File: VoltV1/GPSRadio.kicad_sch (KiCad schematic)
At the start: 13 parts, among them J3 Conn_Coaxial, J4 Conn_Coaxial, U3 MAX-M10S-00B, U9 E22-900M30S

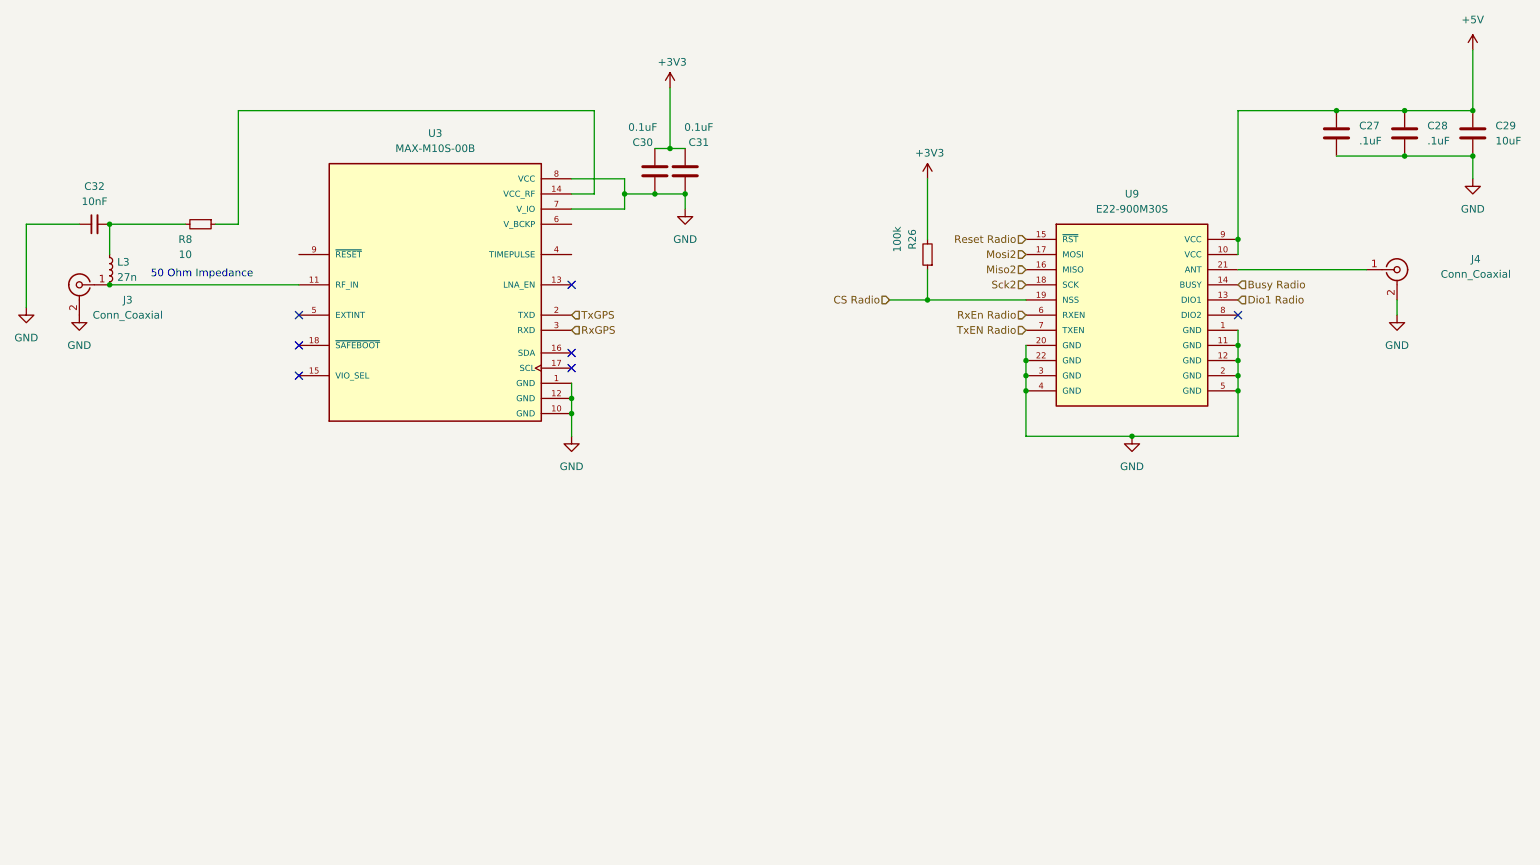
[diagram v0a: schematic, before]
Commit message: updates to schematic
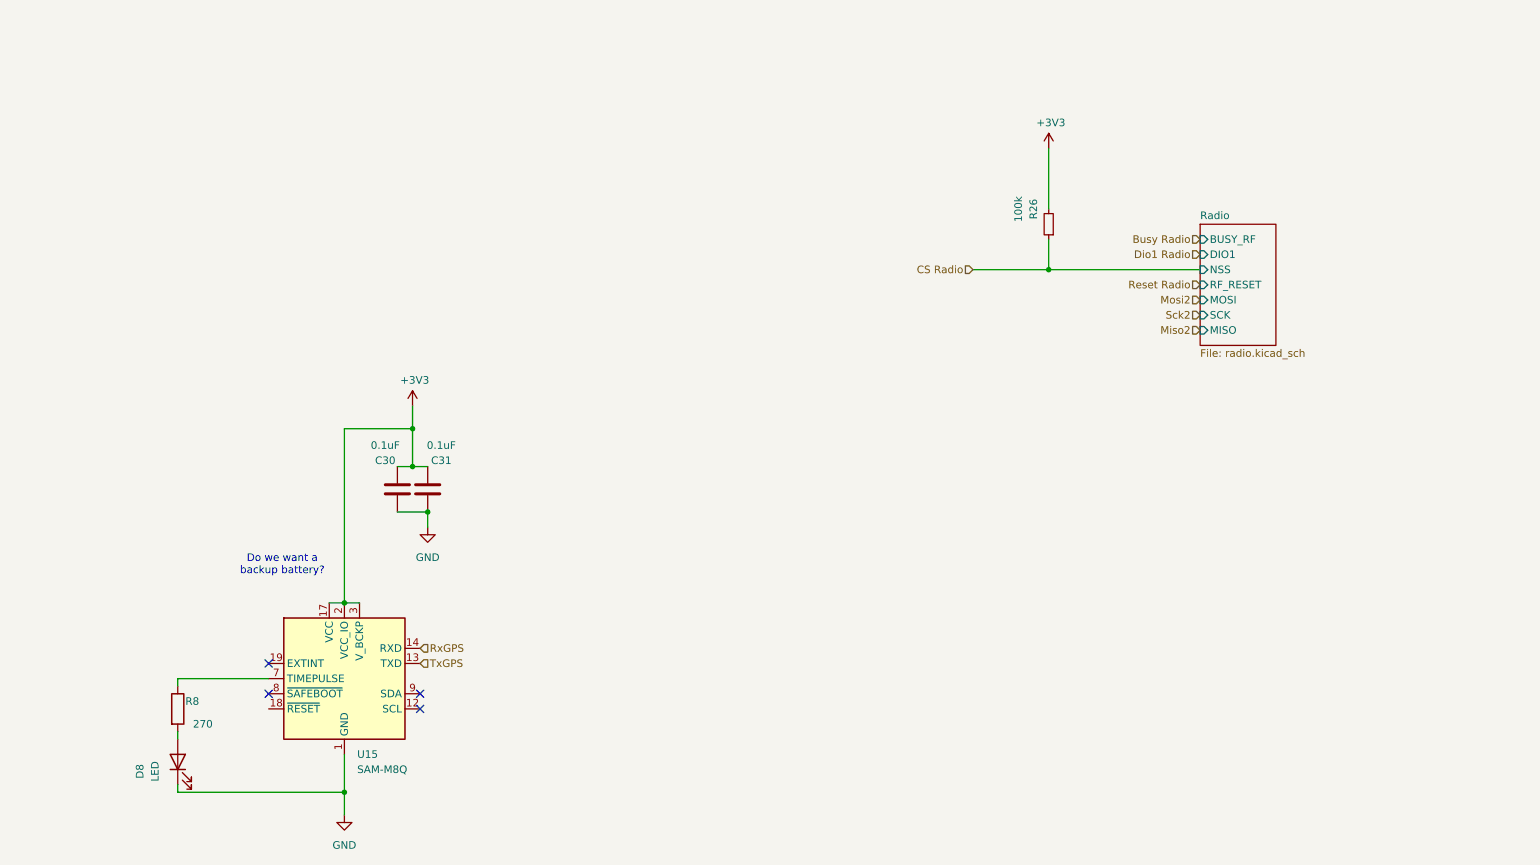
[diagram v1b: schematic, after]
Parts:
- removed C27, C28: .1uF, Capacitor_SMD:C_0603_1608Metric, symbol Device:C
- removed C29: 10uF, Capacitor_SMD:C_0603_1608Metric, symbol Device:C
- removed C32: 10nF, Capacitor_SMD:C_0603_1608Metric, symbol Device:C_Small
- removed J3, J4: Conn_Coaxial, Connector_Coaxial:SMA_Molex_73251-1153_EdgeMount_Horizontal, symbol Connector:Conn_Coaxial
- removed L3: 27n, Inductor_SMD:L_0603_1608Metric, symbol Device:L_Small
- removed R8: 10, Resistor_SMD:R_0603_1608Metric, symbol Device:R_Small
- removed U3: MAX-M10S-00B, VOLTV1:XCVR_MAX-M10S-00B, symbol VOLTV1:MAX-M10S-00B
- removed U9: E22-900M30S, VOLTV1:XCVR_E22-900M30S, symbol VOLTV1:E22-900M30S
- added D8: LED, LED_SMD:LED_0603_1608Metric, symbol Device:LED
- added R8: 270, Resistor_SMD:R_0603_1608Metric, symbol Device:R
- added U15: SAM-M8Q, RF_GPS:ublox_SAM-M8Q, symbol RF_GPS:SAM-M8Q
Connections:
- net +3V3: now also U15.17 (VCC), U15.2 (VCC_IO), U15.3 (V_BCKP)
- net GND: now also D8.1 (K), U15.1 (GND), U15.10 (GND), U15.11 (GND), U15.15 (GND), U15.16 (GND), U15.20 (GND), U15.4 (GND), U15.5 (GND), U15.6 (GND)
- net RxGPS: now also U15.14 (RXD)
- net TxGPS: now also U15.13 (TXD)
- new net: R8.1, U15.7 (TIMEPULSE)
- new net: D8.2 (A), R8.2
- no-connect marks 7 -> 4
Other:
- added sheet Radio (radio.kicad_sch)
- note added: "Do we want a backup battery?"
- note removed: "50 Ohm Impedance"
- moved on the sheet: C30, C31, R26

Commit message: schematic updates
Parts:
- C30, C31: footprint Capacitor_SMD:C_0603_1608Metric -> Capacitor_SMD:C_0402_1005Metric
- R26, R8: footprint Resistor_SMD:R_0603_1608Metric -> Resistor_SMD:R_0402_1005Metric
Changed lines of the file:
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@@
 			)
 		)
-		(property "Footprint" "Resistor_SMD:R_0603_1608Metric"
+		(property "Footprint" "Resistor_SMD:R_0402_1005Metric"
 			(at 42.672 152.4 90)
 			(effects
@@
 			)
 		)
-		(property "Footprint" "Capacitor_SMD:C_0603_1608Metric"
+		(property "Footprint" "Capacitor_SMD:C_0402_1005Metric"
 			(at 85.3948 111.76 0)
 			(effects
@@
 			)
 		)
-		(property "Footprint" "Capacitor_SMD:C_0603_1608Metric"
+		(property "Footprint" "Capacitor_SMD:C_0402_1005Metric"
 			(at 80.3148 111.76 0)
 			(effects
@@
 			)
 		)
-		(property "Footprint" "Resistor_SMD:R_0603_1608Metric"
+		(property "Footprint" "Resistor_SMD:R_0402_1005Metric"
 			(at 190.5 71.12 0)
 			(effects
